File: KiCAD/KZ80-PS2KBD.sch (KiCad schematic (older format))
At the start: 23 parts, among them J1 232C(DEBUG), J2 PS/2 KB, J3 SBC8080 BUS, J4 ADR-JP2, J5 ADR-JP1, J6 ICSP, J7 CON-A, U1 74HC139, U2 74HC00, U3 8255, U4 ATmega328P-PU

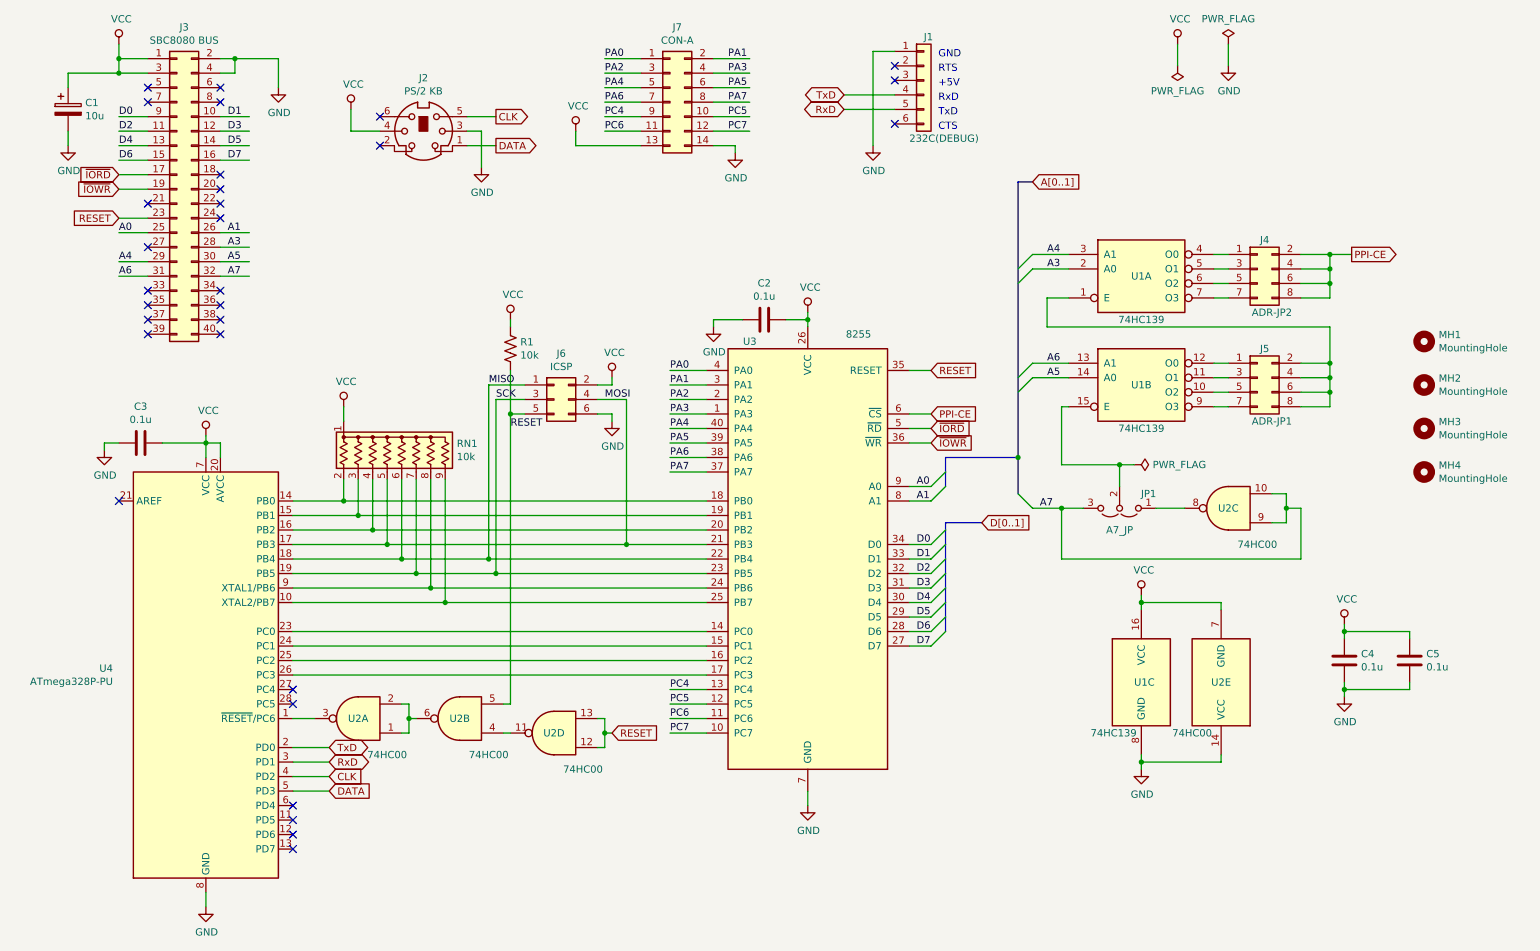
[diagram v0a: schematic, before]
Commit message: REV1基板製造用ガーバーデータ出力版
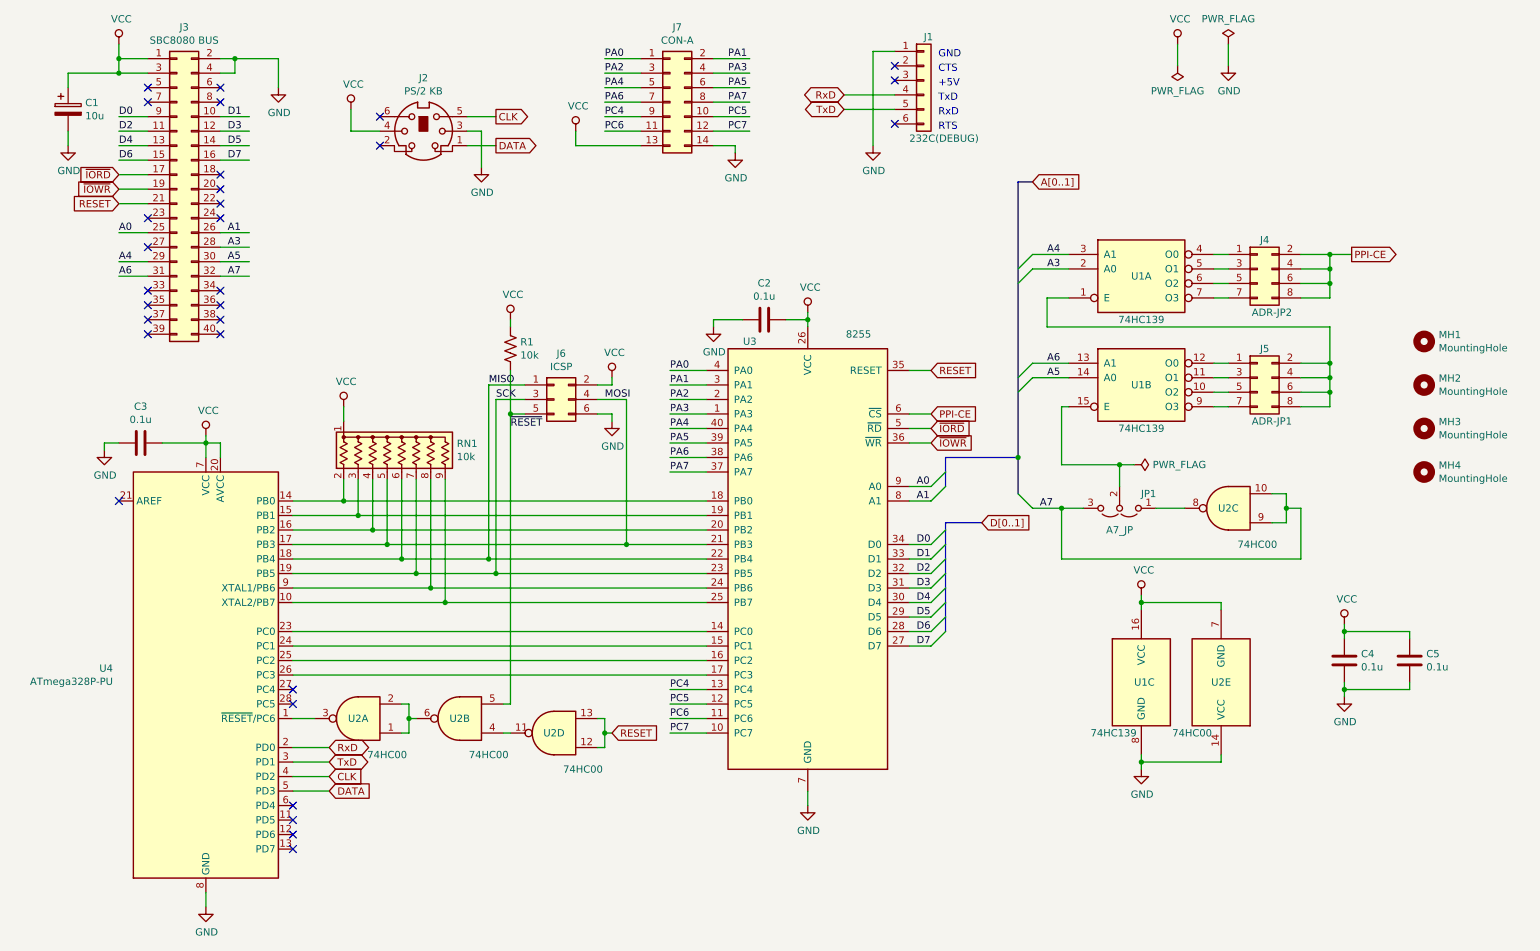
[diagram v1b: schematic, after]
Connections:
- net labels added: ~RESET
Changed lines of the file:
@@
 Wire Wire Line
 	1600 2300 1400 2300
-NoConn ~ 1600 2400
-Text GLabel 1400 2500 0    50   Input ~ 0
+Text GLabel 1400 2400 0    50   Input ~ 0
 RESET
 Wire Wire Line
-	1400 2500 1600 2500
+	1400 2400 1600 2400
 NoConn ~ 2100 2200
 NoConn ~ 2100 2300
@@
 Text Notes 7050 1400 0    50   ~ 0
 GND
-Text Notes 7050 1500 0    50   ~ 0
+Text Notes 7050 1900 0    50   ~ 0
 RTS
 Text Notes 7050 1600 0    50   ~ 0
 +5V
+Text Notes 7050 1800 0    50   ~ 0
+RxD
 Text Notes 7050 1700 0    50   ~ 0
-RxD
-Text Notes 7050 1800 0    50   ~ 0
 TxD
-Text Notes 7050 1900 0    50   ~ 0
+Text Notes 7050 1500 0    50   ~ 0
 CTS
 NoConn ~ 6750 1850
@@
 Wire Wire Line
 	6600 1350 6600 2000
+Text GLabel 6400 1750 0    50   BiDi ~ 0
+TxD
+Wire Wire Line
+	6400 1650 6750 1650
 Text GLabel 6400 1650 0    50   BiDi ~ 0
+RxD
+Wire Wire Line
+	6400 1750 6750 1750
+Text GLabel 2850 6250 2    50   BiDi ~ 0
 TxD
-Wire Wire Line
-	6400 1650 6750 1650
-Text GLabel 6400 1750 0    50   BiDi ~ 0
-RxD
-Wire Wire Line
-	6400 1750 6750 1750
 Text GLabel 2850 6150 2    50   BiDi ~ 0
-TxD
-Text GLabel 2850 6250 2    50   BiDi ~ 0
 RxD
 Wire Wire Line
@@
 SCK
 Text Label 4100 3950 0    50   ~ 0
-RESET
+~RESET
 Text Label 4750 3750 0    50   ~ 0
 MOSI
@@
 Wire Wire Line
 	5650 2000 5650 2050
-Wire Bus Line
-	7100 4150 7100 4350
-Wire Bus Line
-	7600 2250 7600 4150
-Wire Bus Line
-	7100 4600 7100 5350
 $Comp
 L Mechanical:MountingHole MH1
@@
 	1    0    0    -1
 $EndComp
+NoConn ~ 1600 2500
+Wire Bus Line
+	7100 4150 7100 4350
+Wire Bus Line
+	7600 2250 7600 4150
+Wire Bus Line
+	7100 4600 7100 5350
 $EndSCHEMATC
